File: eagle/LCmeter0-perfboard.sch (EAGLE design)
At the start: 25 parts, among them IC1 PIC16F876A-X/SP, K2 DS2Y, Q1 20MHz, Q2 BC548, SW1 SPST, SW2 DPDT

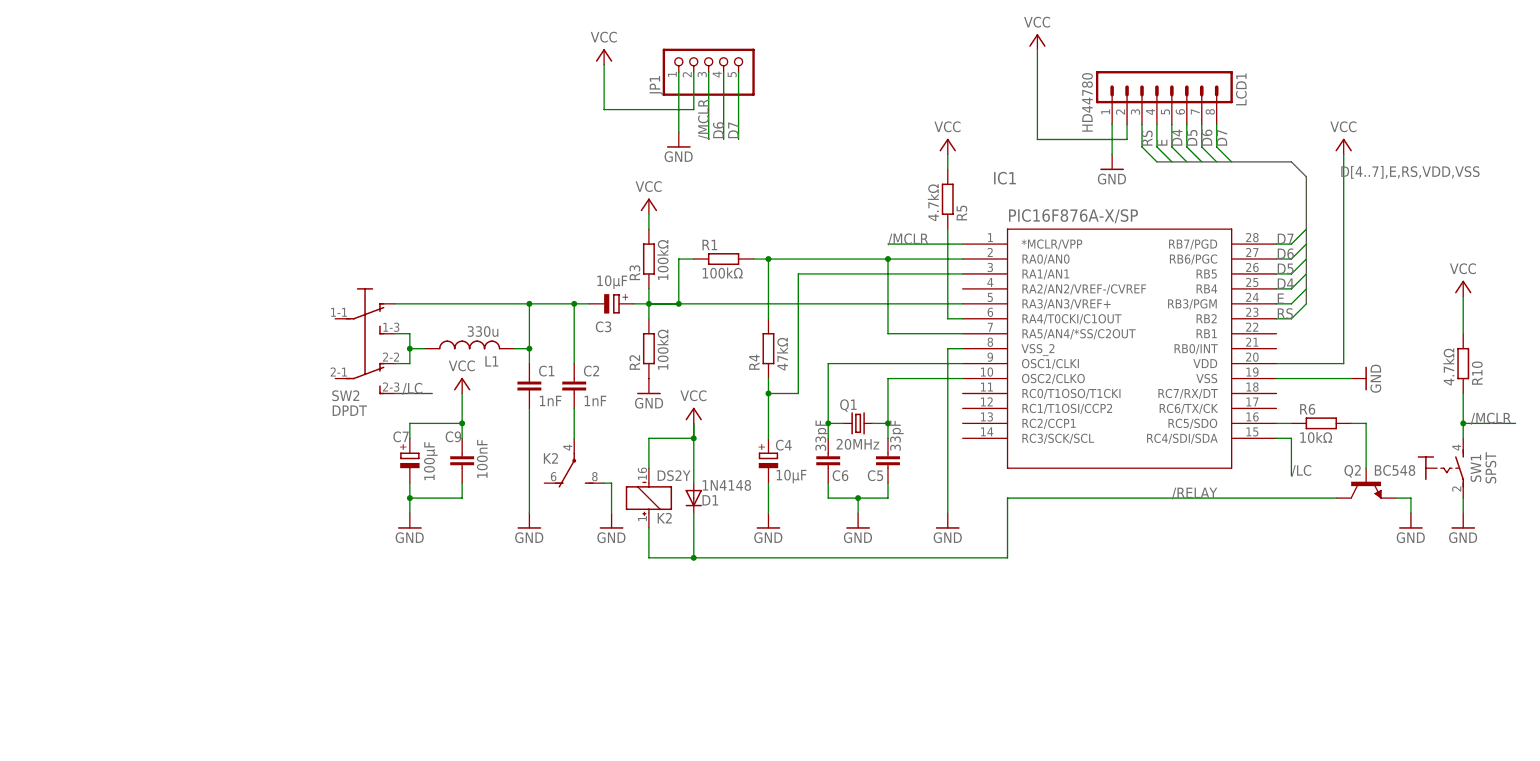
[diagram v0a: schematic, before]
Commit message: ...
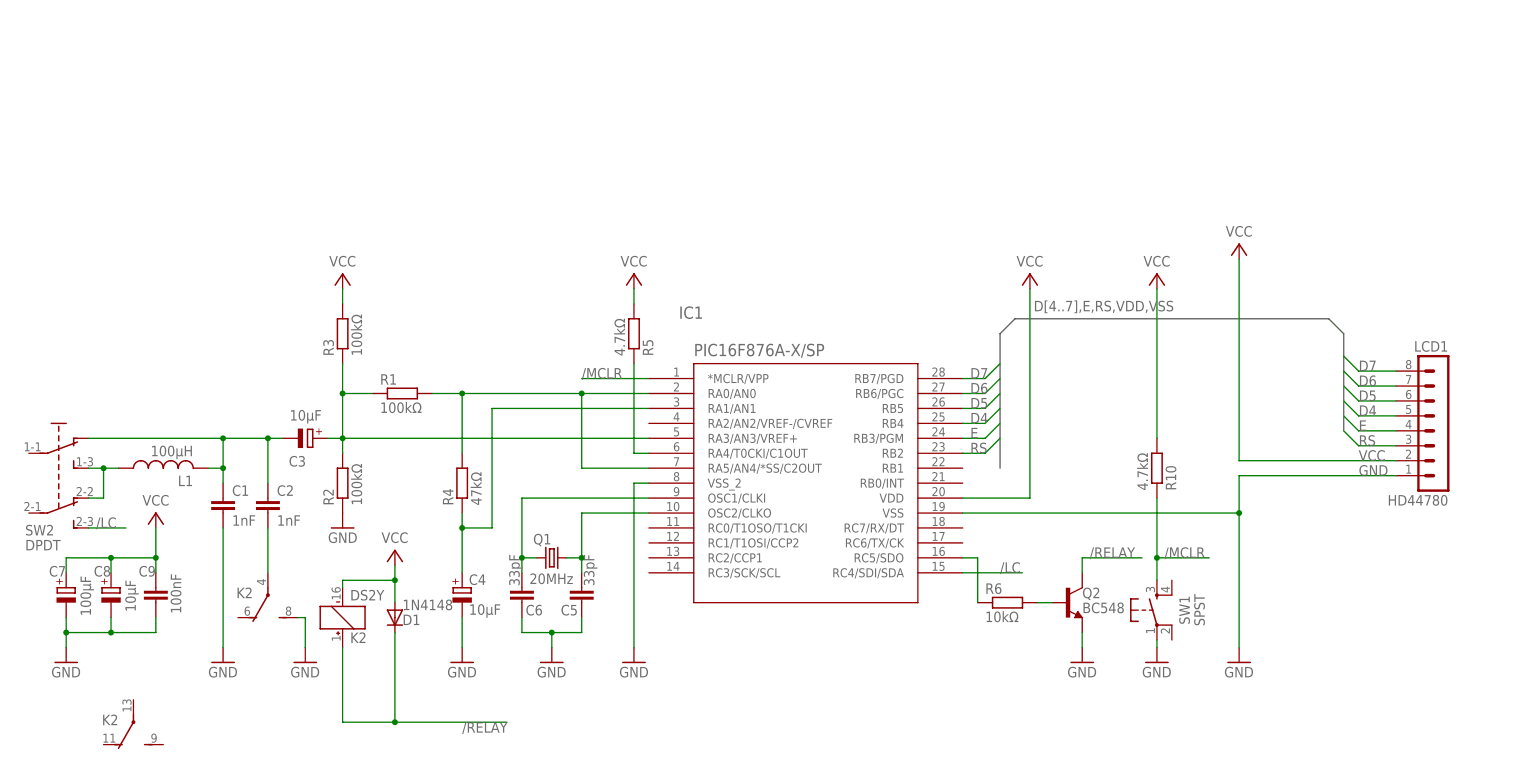
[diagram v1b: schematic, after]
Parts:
- removed JP1: (no value), pinhead:PINHD-1X5
- added C8: 10μF, rcl:CPOL-EUE2.5-5
- C3, C4: device rcl:CPOL-EUE2.5-5 -> rcl:CPOL-EUE5-4
- C5, C6: device rcl:C-EU025-024X044 -> rcl:C-EU050-024X044
- L1: value 330u -> 100μH
- R1: device rcl:R-EU_0207/10 -> resistor:R-EU_0204/2V
- R10: device resistor:R-EU_0207/10 -> resistor:R-EU_0204/2V
- R5: device resistor:R-EU_0204/7 -> resistor:R-EU_0204/2V
- R6: device resistor:R-EU_0204/7 -> rcl:R-EU_0207/10
- SW1: device lc-meter:PB-5-2 -> lc-meter:PB-SPST
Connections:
- net /MCLR: no longer JP1.3
- net D6: no longer JP1.4
- net D7: no longer JP1.5
- net GND: now also C8.-; no longer JP1.1
- net VCC: now also C8.+; no longer JP1.2
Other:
- moved on the sheet: C1, C2, C3, C4, C5, C6, C7, C9, D1, IC1, K2, L1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

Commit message: ...
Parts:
- R1: device resistor:R-EU_0204/2V -> rcl:R-EU_0204/7
- R10, R5: device resistor:R-EU_0204/2V -> resistor:R-EU_0207/10
- R6: device rcl:R-EU_0207/10 -> resistor:R-EU_0204/2V
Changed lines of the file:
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@@
 <?xml version="1.0" encoding="utf-8"?>
 <!DOCTYPE eagle SYSTEM "eagle.dtd">
-<eagle version="7.2.0">
+<eagle version="7.3.0">
 <drawing>
 <settings>
@@
 <parts>
 <part name="IC1" library="lc-meter" deviceset="PIC16F876A-X/SP" device=""/>
-<part name="R1" library="resistor" deviceset="R-EU_" device="0204/2V" value="100kΩ"/>
+<part name="R1" library="rcl" deviceset="R-EU_" device="0204/7" value="100kΩ"/>
 <part name="R2" library="resistor" deviceset="R-EU_" device="0204/2V" value="100kΩ"/>
 <part name="R3" library="resistor" deviceset="R-EU_" device="0204/2V" value="100kΩ"/>
 <part name="R4" library="resistor" deviceset="R-EU_" device="0204/2V" value="47kΩ"/>
-<part name="R10" library="resistor" deviceset="R-EU_" device="0204/2V" value="4.7kΩ"/>
+<part name="R10" library="resistor" deviceset="R-EU_" device="0207/10" value="4.7kΩ"/>
 <part name="C1" library="rcl" deviceset="C-EU" device="050-024X044" value="1nF"/>
 <part name="C2" library="rcl" deviceset="C-EU" device="050-024X044" value="1nF"/>
@@
 <part name="P+4" library="supply1" deviceset="VCC" device=""/>
 <part name="GND12" library="supply1" deviceset="GND" device=""/>
-<part name="R5" library="resistor" deviceset="R-EU_" device="0204/2V" value="4.7kΩ"/>
+<part name="R5" library="resistor" deviceset="R-EU_" device="0207/10" value="4.7kΩ"/>
 <part name="P+5" library="supply1" deviceset="VCC" device=""/>
 <part name="GND14" library="supply1" deviceset="GND" device=""/>
@@
 <part name="Q2" library="transistor-npn" deviceset="BC548*" device=""/>
 <part name="GND8" library="supply1" deviceset="GND" device=""/>
-<part name="R6" library="rcl" deviceset="R-EU_" device="0207/10" value="10kΩ"/>
+<part name="R6" library="resistor" deviceset="R-EU_" device="0204/2V" value="10kΩ"/>
 <part name="LCD1" library="con-lstb" deviceset="MA08-1" device="" value="HD44780"/>
 <part name="P+7" library="supply1" deviceset="VCC" device=""/>

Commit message: ...
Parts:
- C4: device rcl:CPOL-EUE5-4 -> rcl:CPOL-EUE2.5-5
- C5, C6: device rcl:C-EU050-024X044 -> rcl:C-EU025-024X044
- R6: device resistor:R-EU_0204/2V -> resistor:R-EU_0204/5
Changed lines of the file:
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@@
 <part name="C2" library="rcl" deviceset="C-EU" device="050-024X044" value="1nF"/>
 <part name="C3" library="rcl" deviceset="CPOL-EU" device="E5-4" value="10μF"/>
-<part name="C4" library="rcl" deviceset="CPOL-EU" device="E5-4" value="10μF"/>
-<part name="C5" library="rcl" deviceset="C-EU" device="050-024X044" value="33pF"/>
-<part name="C6" library="rcl" deviceset="C-EU" device="050-024X044" value="33pF"/>
+<part name="C4" library="rcl" deviceset="CPOL-EU" device="E2.5-5" value="10μF"/>
+<part name="C5" library="rcl" deviceset="C-EU" device="025-024X044" value="33pF"/>
+<part name="C6" library="rcl" deviceset="C-EU" device="025-024X044" value="33pF"/>
 <part name="C7" library="rcl" deviceset="CPOL-EU" device="E2.5-6" value="100μF"/>
 <part name="C8" library="rcl" deviceset="CPOL-EU" device="E2.5-5" value="10μF"/>
@@
 <part name="Q2" library="transistor-npn" deviceset="BC548*" device=""/>
 <part name="GND8" library="supply1" deviceset="GND" device=""/>
-<part name="R6" library="resistor" deviceset="R-EU_" device="0204/2V" value="10kΩ"/>
+<part name="R6" library="resistor" deviceset="R-EU_" device="0204/5" value="10kΩ"/>
 <part name="LCD1" library="con-lstb" deviceset="MA08-1" device="" value="HD44780"/>
 <part name="P+7" library="supply1" deviceset="VCC" device=""/>

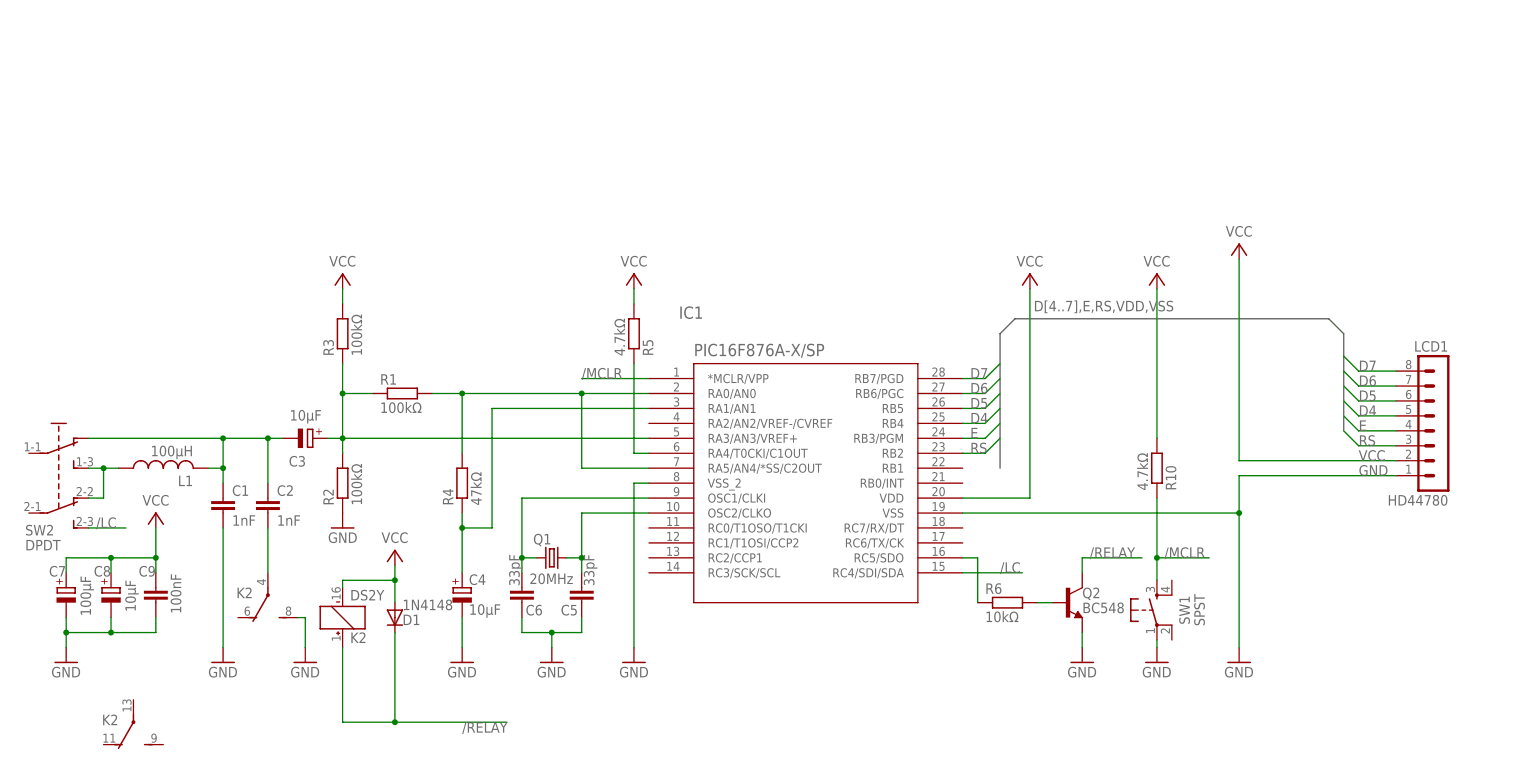
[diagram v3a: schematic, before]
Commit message: ...
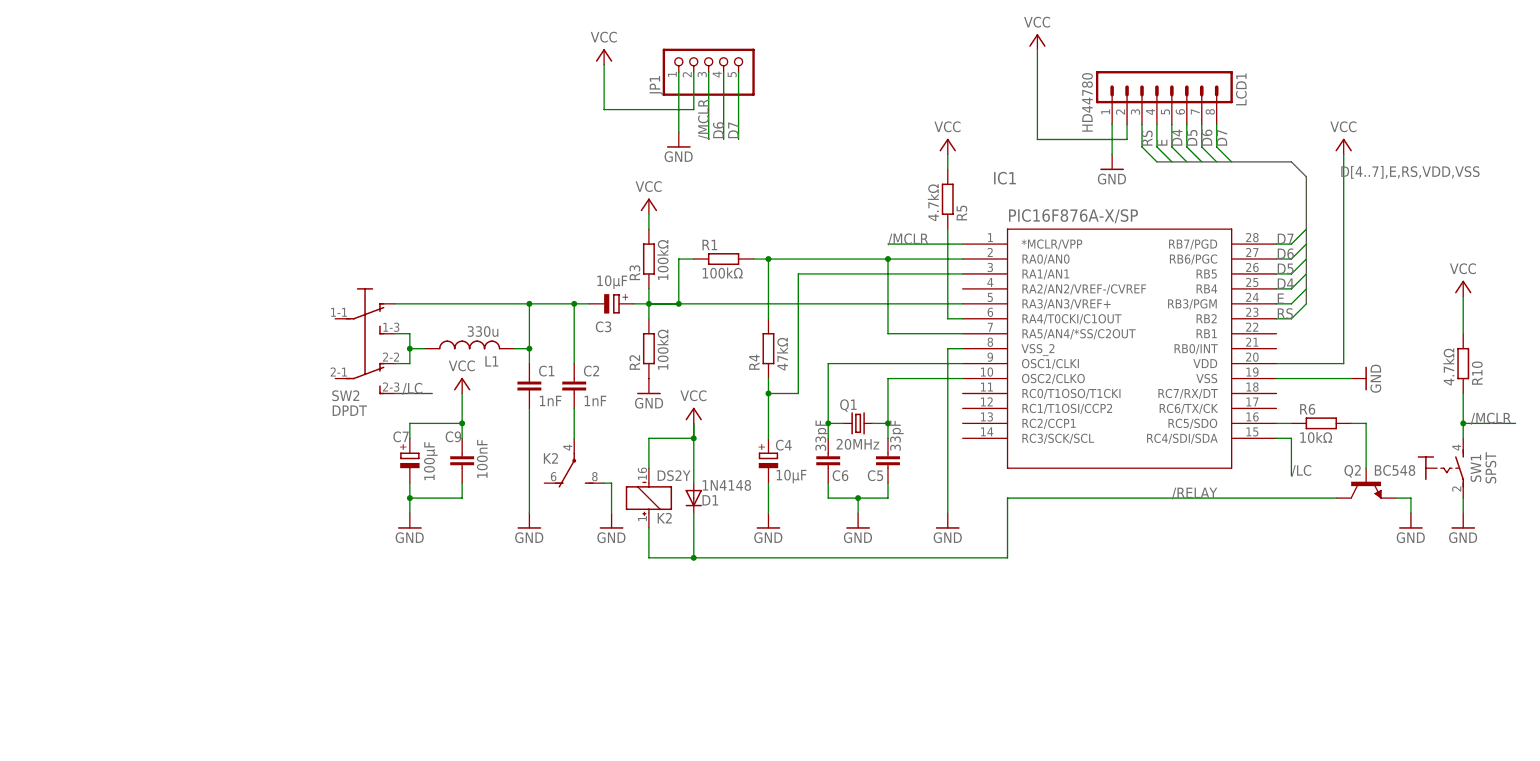
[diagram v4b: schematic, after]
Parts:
- removed C8: 10μF, rcl:CPOL-EUE2.5-5
- added JP1: (no value), pinhead:PINHD-1X5
- C3: device rcl:CPOL-EUE5-4 -> rcl:CPOL-EUE2.5-5
- L1: value 100μH -> 330u
- R1: device rcl:R-EU_0204/7 -> rcl:R-EU_0207/10
- R6: device resistor:R-EU_0204/5 -> resistor:R-EU_0204/7
- SW1: device lc-meter:PB-SPST -> lc-meter:PB-5-2
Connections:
- net /MCLR: now also JP1.3
- net D6: now also JP1.4
- net D7: now also JP1.5
- net GND: now also JP1.1; no longer C8.-
- net VCC: now also JP1.2; no longer C8.+
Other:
- moved on the sheet: C1, C2, C3, C4, C5, C6, C7, C9, D1, IC1, K2, L1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
